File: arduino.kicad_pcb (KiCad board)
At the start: 2 copper layers, 101.6 x 53.3 mm, 82 parts, among them J1 USB_A, J10 7SEL, J11 PA, J12 PB, J13 PC, J14 PD, J15 MICROWIRE, J16 ISP, J17 POWER, J18 USB_B_Micro, J2 NE7555, J3 7SEG, J4 DCJ0202, J5 PWR, J6 UART, J7 PG, J8 PF, J9 PE, Q1 FDN340P, Q2 2N3903, SW1 OP, SW2 PRG, SW3 RST, U1 ICM7555, U2 LM358, U3 FT232RL, U4 MT30361, U5 MC33269D-5.0, U6 ATmega128-16AU, U7 M93C86-WMN6TP, Y1 Crystal

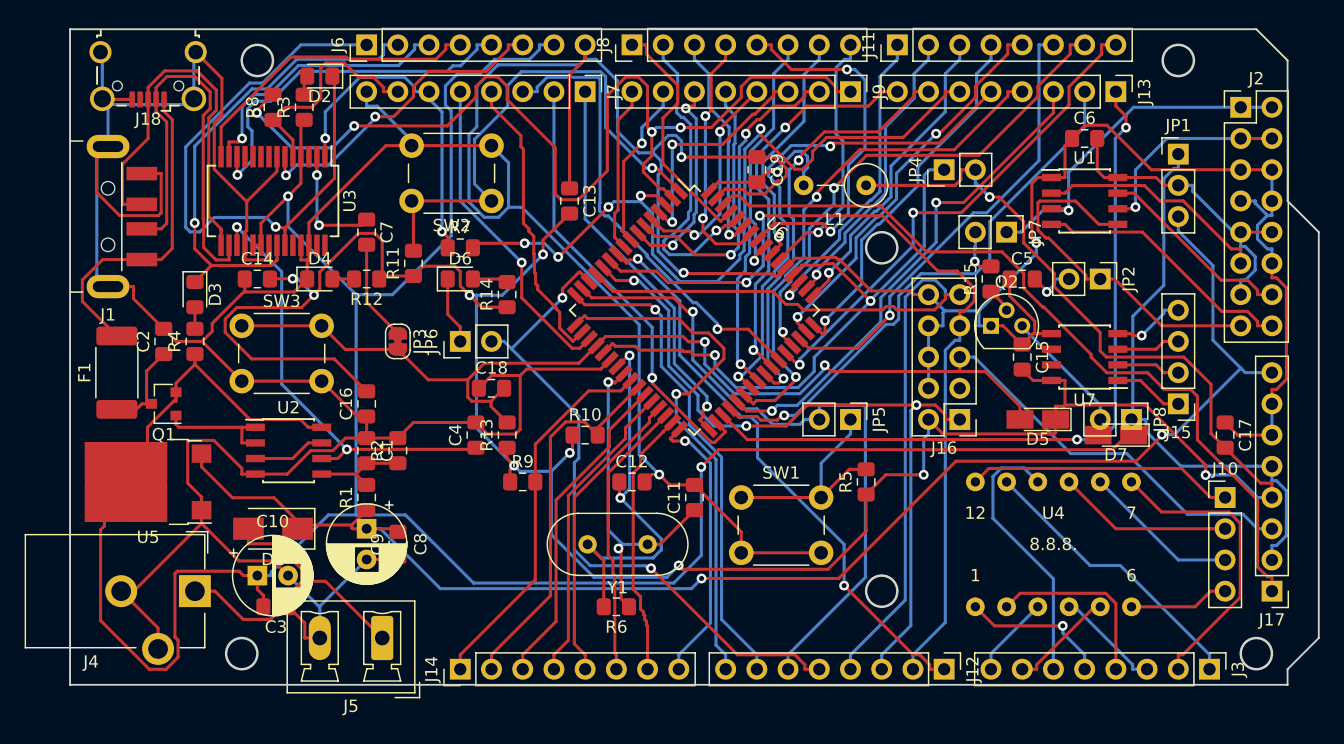
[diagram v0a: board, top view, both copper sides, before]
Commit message: Routed
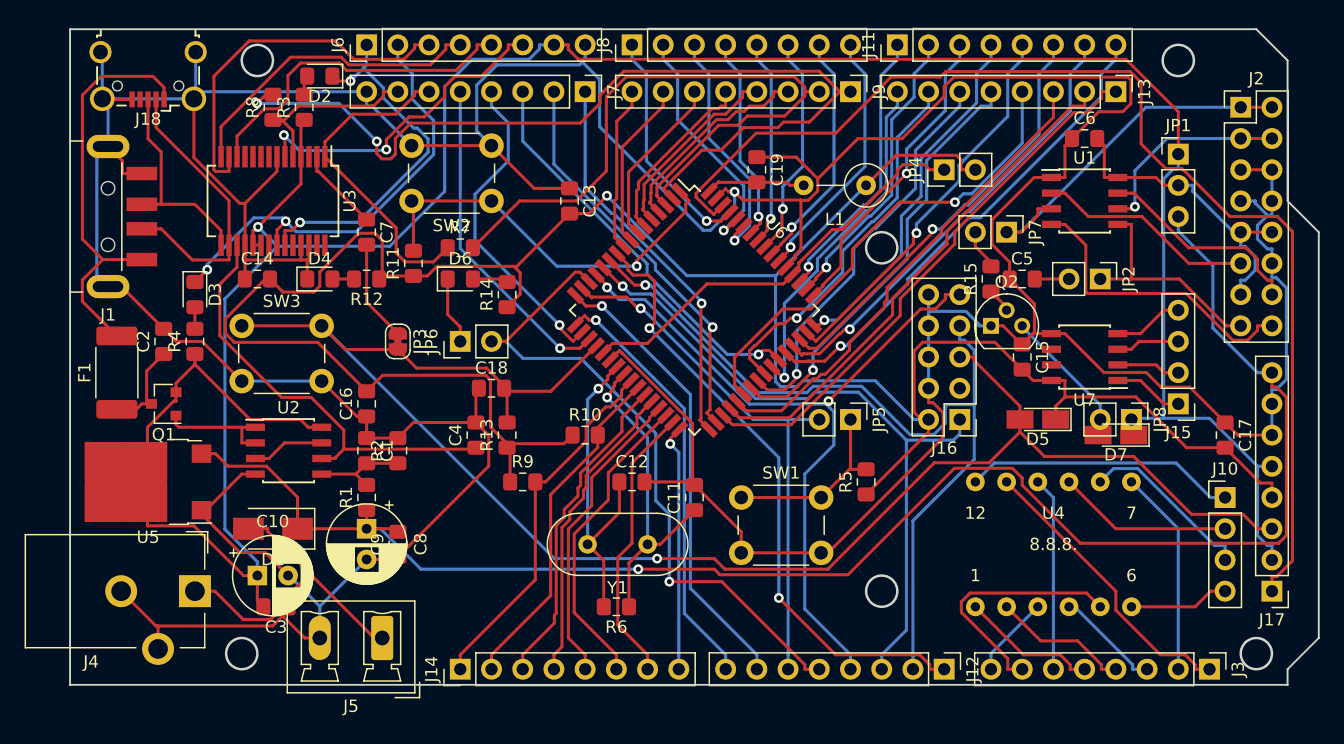
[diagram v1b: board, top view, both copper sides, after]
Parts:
- C2, C4: value C 100n -> 100n
- C3, C7: value C -> 0.1u
- F1: value Fuse -> 0.5RST
- JP3: value Jumper -> AVR
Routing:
- net +5V: track 273.9 -> 229.4 mm, vias 2 -> 1
- net NEGND: track 488.9 -> 448.7 mm, vias 4 -> 1
- net aref: track 65.1 -> 94.6 mm
- net VCC: track 226.4 -> 199.2 mm, vias 10 -> 1
- net reset: track 112.8 -> 137.5 mm, vias 2 -> 1
- net cbus0: track 49.3 -> 29.8 mm, vias 1 -> 2
- net vin: track 119.3 -> 135.2 mm, vias 2 -> 1
- net Net-(J13-Pad1): track 61.0 -> 45.2 mm, vias 2 -> 0
- net Net-(JP4-Pad1): track 49.5 -> 34.7 mm, vias 2 -> 0
- net Net-(J1-Pad3): track 32.0 -> 17.5 mm
- net Net-(J8-Pad5): track 30.4 -> 16.8 mm, vias 2 -> 1
- net Net-(J1-Pad2): track 35.5 -> 23.7 mm
- net Net-(J3-Pad7): track 8.67 -> 20.3 mm
- net pb5: track 55.3 -> 44.1 mm
- net NECTRLV: track 29.5 -> 18.6 mm
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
